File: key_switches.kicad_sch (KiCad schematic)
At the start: 78 parts, among them SW1 SW_Push, SW10 SW_Push, SW11 SW_Push, SW12 SW_Push, SW13 SW_Push, SW14 SW_Push, SW15 SW_Push, SW16 SW_Push, SW17 SW_Push, SW18 SW_Push, SW19 SW_Push, SW2 SW_Push, SW20 SW_Push, SW21 SW_Push, SW22 SW_Push, SW23 SW_Push, SW24 SW_Push, SW25 SW_Push, SW26 SW_Push, SW27 SW_Push, SW28 SW_Push, SW29 SW_Push, SW3 SW_Push, SW30 SW_Push, SW31 SW_Push, SW32 SW_Push, SW33 SW_Push, SW34 SW_Push, SW35 SW_Push, SW36 SW_Push, SW37 SW_Push, SW38 SW_Push, SW39 SW_Push, SW4 SW_Push, SW5 SW_Push, SW6 SW_Push, SW7 SW_Push, SW8 SW_Push, SW9 SW_Push

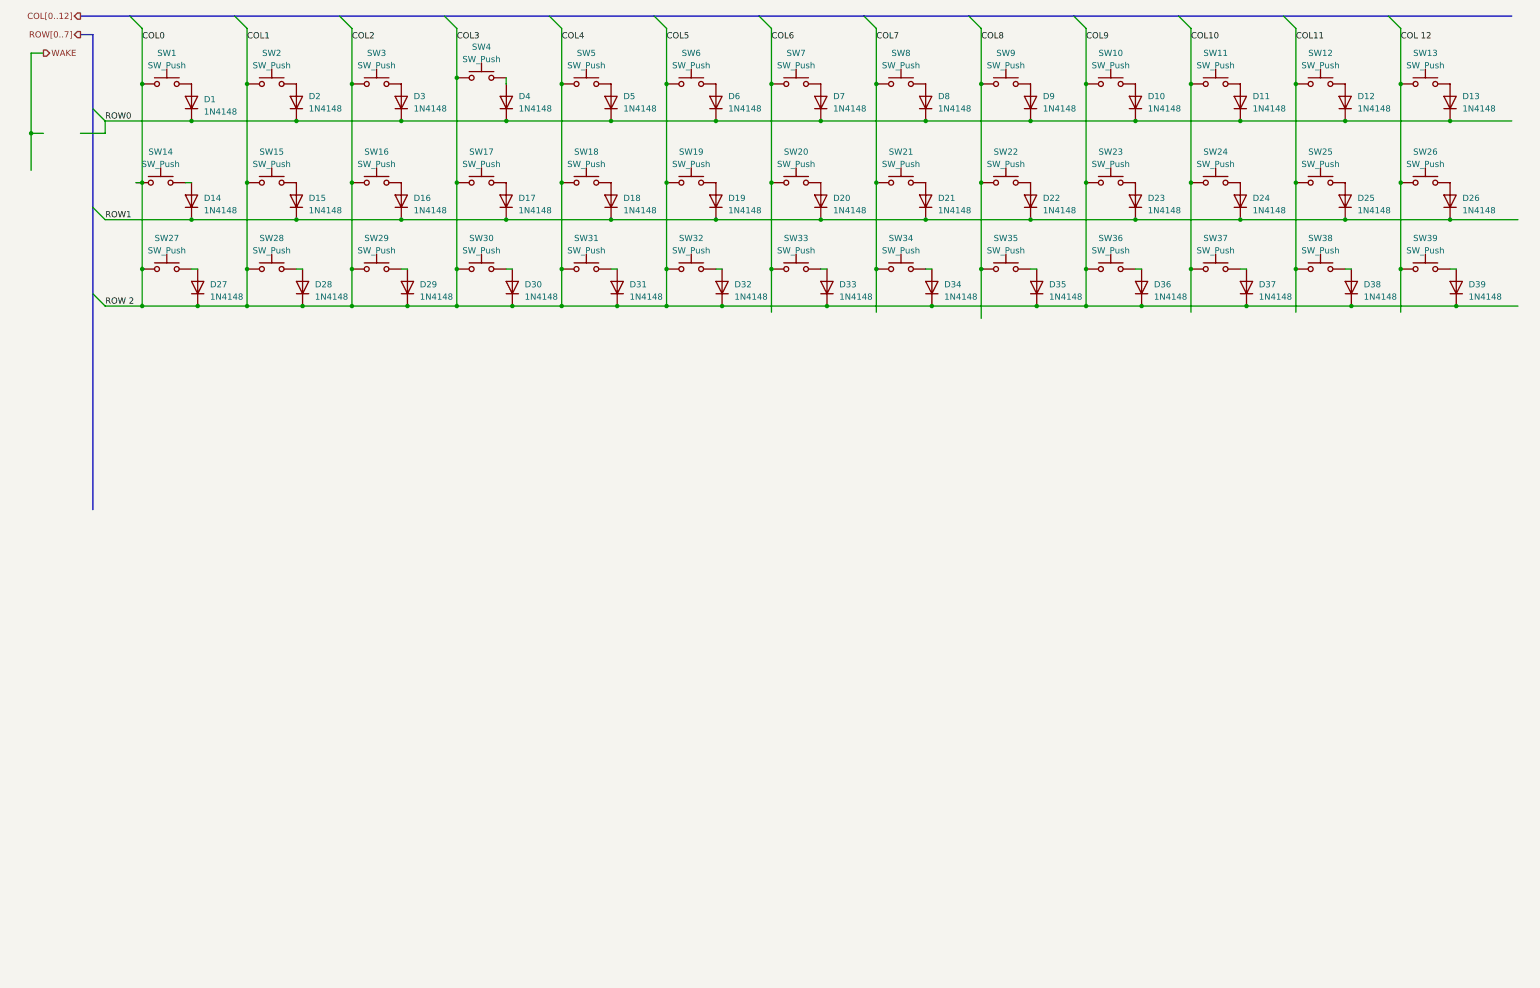
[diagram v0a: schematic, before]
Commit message: SHOULD BE DONE!!!!!!!
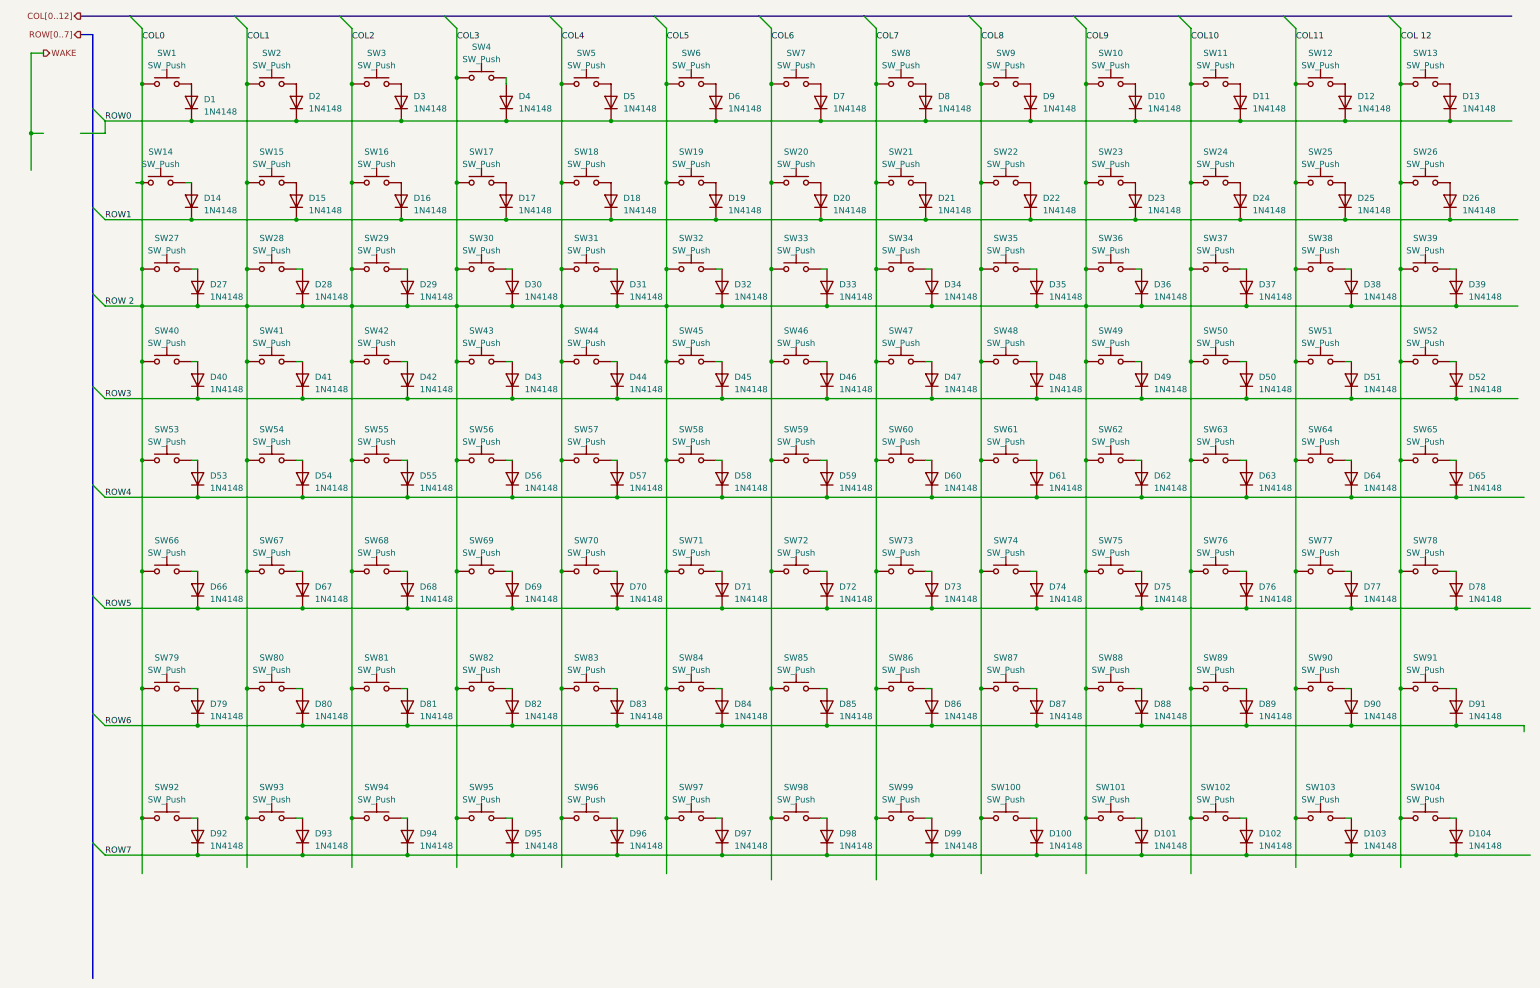
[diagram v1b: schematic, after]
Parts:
- added D100, D101, D102, D103, D104, D40, D41, D42, D43, D44, D45, D46, D47, D48, D49, D50, D51, D52, D53, D54, D55, D56, D57, D58, D59, D60, D61, D62, D63, D64, D65, D66, D67, D68, D69, D70, D71, D72, D73, D74, D75, D76, D77, D78, D79, D80, D81, D82, D83, D84, D85, D86, D87, D88, D89, D90, D91, D92, D93, D94, D95, D96, D97, D98, D99: 1N4148, Diode_THT:D_DO-35_SOD27_P7.62mm_Horizontal, symbol Diode:1N4148
- added SW100, SW101, SW102, SW103, SW104, SW40, SW41, SW42, SW43, SW44, SW45, SW46, SW47, SW48, SW49, SW50, SW51, SW52, SW53, SW54, SW55, SW56, SW57, SW58, SW59, SW60, SW61, SW62, SW63, SW64, SW65, SW66, SW67, SW68, SW69, SW70, SW71, SW72, SW73, SW74, SW75, SW76, SW77, SW78, SW79, SW80, SW81, SW82, SW83, SW84, SW85, SW86, SW87, SW88, SW89, SW90, SW91, SW92, SW93, SW94, SW95, SW96, SW97, SW98, SW99: SW_Push, symbol Switch:SW_Push
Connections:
- net COL 12: now also SW104.1, SW52.1, SW65.1, SW78.1, SW91.1
- net COL0: now also SW101.1, SW40.1, SW41.1, SW42.1, SW43.1, SW44.1, SW45.1, SW49.1, SW53.1, SW54.1, SW55.1, SW56.1, SW57.1, SW58.1, SW62.1, SW66.1, SW67.1, SW68.1, SW69.1, SW70.1, SW71.1, SW75.1, SW79.1, SW80.1, SW81.1, SW82.1, SW83.1, SW84.1, SW88.1, SW92.1, SW93.1, SW94.1, SW95.1, SW96.1, SW97.1
- net COL10: now also SW102.1, SW50.1, SW63.1, SW76.1, SW89.1
- net COL11: now also SW103.1, SW51.1, SW64.1, SW77.1, SW90.1
- net COL6: now also SW46.1, SW59.1, SW72.1, SW85.1, SW98.1
- net COL7: now also SW47.1, SW60.1, SW73.1, SW86.1, SW99.1
- net COL8: now also SW100.1, SW48.1, SW61.1, SW74.1, SW87.1
- new net: D74.2 (A), SW74.2
- new net: D102.2 (A), SW102.2
- new net: D44.2 (A), SW44.2
- new net: D84.2 (A), SW84.2
- new net: D69.2 (A), SW69.2
- new net: D95.2 (A), SW95.2
- new net: D76.2 (A), SW76.2
- new net: D48.2 (A), SW48.2
- new net: D83.2 (A), SW83.2
- new net: D86.2 (A), SW86.2
- new net: D81.2 (A), SW81.2
- new net: D66.2 (A), SW66.2
- new net: D71.2 (A), SW71.2
- new net: D103.2 (A), SW103.2
- new net: D99.2 (A), SW99.2
- new net: D51.2 (A), SW51.2
- new net: D58.2 (A), SW58.2
- new net: D87.2 (A), SW87.2
- new net: D63.2 (A), SW63.2
- new net: D65.2 (A), SW65.2
- new net: D60.2 (A), SW60.2
- new net: D46.2 (A), SW46.2
- new net: D42.2 (A), SW42.2
- new net: D104.2 (A), SW104.2
- new net: D67.2 (A), SW67.2
- new net: D101.2 (A), SW101.2
- new net: D68.2 (A), SW68.2
- new net: D89.2 (A), SW89.2
- new net: D94.2 (A), SW94.2
- new net: D79.2 (A), SW79.2
- new net: D97.2 (A), SW97.2
- new net: D49.2 (A), SW49.2
- new net: D62.2 (A), SW62.2
- new net: D70.2 (A), SW70.2
- new net: D82.2 (A), SW82.2
- new net: D93.2 (A), SW93.2
- new net: D80.2 (A), SW80.2
- new net: D57.2 (A), SW57.2
- new net: D56.2 (A), SW56.2
- new net: D43.2 (A), SW43.2
- new net: D59.2 (A), SW59.2
- new net: D77.2 (A), SW77.2
- new net: D50.2 (A), SW50.2
- new net: D45.2 (A), SW45.2
- new net: D75.2 (A), SW75.2
- new net: D64.2 (A), SW64.2
- new net: D73.2 (A), SW73.2
- new net: D78.2 (A), SW78.2
- new net: D41.2 (A), SW41.2
- new net: D88.2 (A), SW88.2
- new net: D96.2 (A), SW96.2
- new net: D52.2 (A), SW52.2
- new net: D40.2 (A), SW40.2
- new net: D61.2 (A), SW61.2
- new net: D54.2 (A), SW54.2
- new net: D98.2 (A), SW98.2
- new net: D55.2 (A), SW55.2
- new net: D72.2 (A), SW72.2
- new net: D100.2 (A), SW100.2
- new net: D47.2 (A), SW47.2
- new net: D90.2 (A), SW90.2
- new net: D85.2 (A), SW85.2
- new net: D92.2 (A), SW92.2
- new net: D91.2 (A), SW91.2
- new net: D53.2 (A), SW53.2
- new net ROW3: D40.1 (K), D41.1 (K), D42.1 (K), D43.1 (K), D44.1 (K), D45.1 (K), D46.1 (K), D47.1 (K), D48.1 (K), D49.1 (K), D50.1 (K), D51.1 (K), D52.1 (K)
- new net ROW4: D53.1 (K), D54.1 (K), D55.1 (K), D56.1 (K), D57.1 (K), D58.1 (K), D59.1 (K), D60.1 (K), D61.1 (K), D62.1 (K), D63.1 (K), D64.1 (K), D65.1 (K)
- new net ROW5: D66.1 (K), D67.1 (K), D68.1 (K), D69.1 (K), D70.1 (K), D71.1 (K), D72.1 (K), D73.1 (K), D74.1 (K), D75.1 (K), D76.1 (K), D77.1 (K), D78.1 (K)
- new net ROW6: D79.1 (K), D80.1 (K), D81.1 (K), D82.1 (K), D83.1 (K), D84.1 (K), D85.1 (K), D86.1 (K), D87.1 (K), D88.1 (K), D89.1 (K), D90.1 (K), D91.1 (K)
- new net ROW7: D100.1 (K), D101.1 (K), D102.1 (K), D103.1 (K), D104.1 (K), D92.1 (K), D93.1 (K), D94.1 (K), D95.1 (K), D96.1 (K), D97.1 (K), D98.1 (K), D99.1 (K)
